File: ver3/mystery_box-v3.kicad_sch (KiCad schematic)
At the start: 3 parts, among them J1 Conn_01x02_Socket, Q1 IRLZ44N

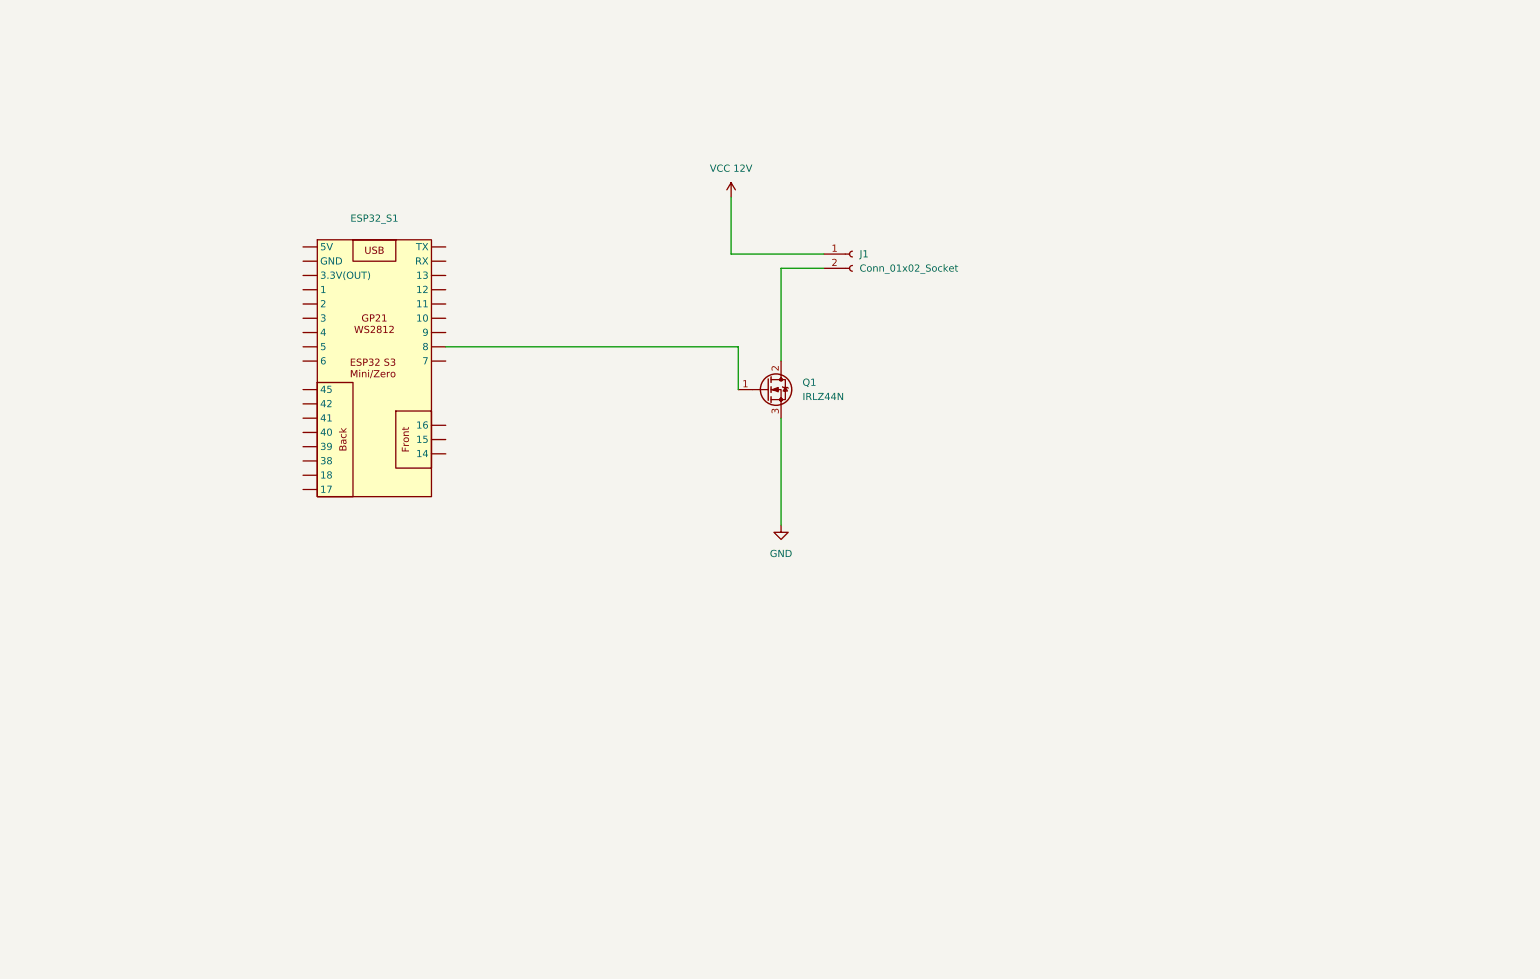
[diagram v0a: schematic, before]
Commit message: first draft v3
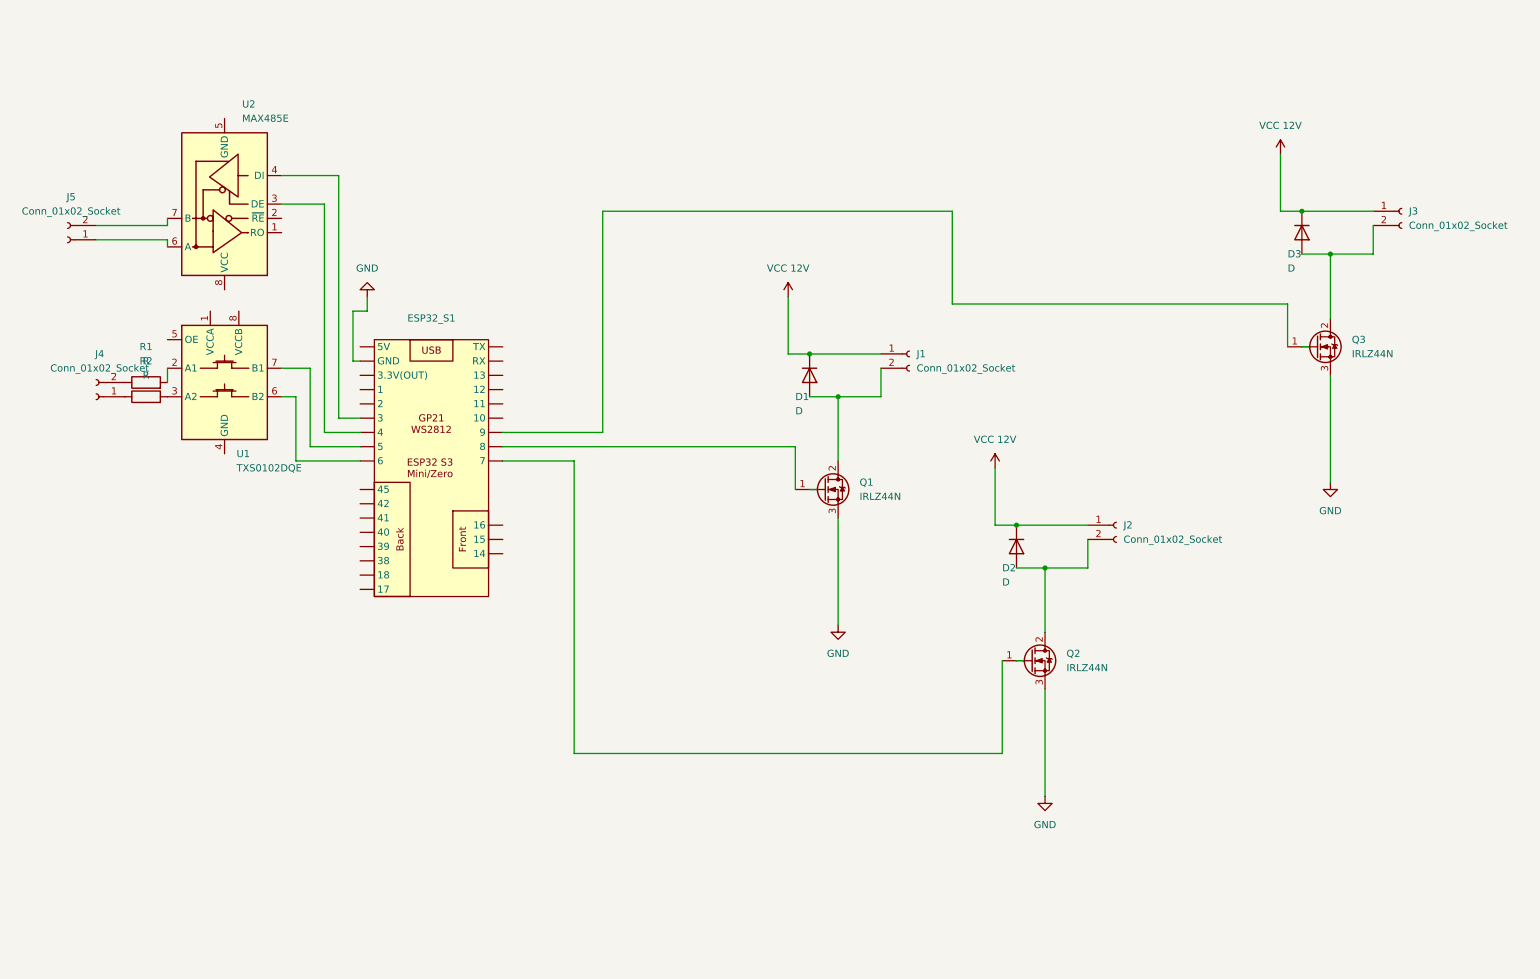
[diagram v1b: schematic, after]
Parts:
- added D1, D2, D3: D, symbol Device:D
- added J2, J3, J4, J5: Conn_01x02_Socket, symbol Connector:Conn_01x02_Socket
- added Q2, Q3: IRLZ44N, Package_TO_SOT_THT:TO-220-3_Vertical, symbol Transistor_FET:IRLZ44N
- added R1, R2: R, symbol Device:R
- added U1: TXS0102DQE, Package_SON:X2SON-8_1.4x1mm_P0.35mm, symbol Logic_LevelTranslator:TXS0102DQE
- added U2: MAX485E, Package_SO:SOIC-8_3.9x4.9mm_P1.27mm, symbol Interface_UART:MAX485E
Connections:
- net GND: now also ESP32_S1. (14), Q2.3 (S), Q3.3 (S)
- net VCC 12V: now also D1.1 (K), D2.1 (K), D3.1 (K), J2.1 (Pin_1), J3.1 (Pin_1)
- net at J1.2 (Pin_2), Q1.2 (D): now also D1.2 (A)
- new net: D3.2 (A), J3.2 (Pin_2), Q3.2 (D)
- new net: J4.1 (Pin_1), R2.1
- new net: R2.2, U1.3 (A2)
- new net: J4.2 (Pin_2), R1.1
- new net: R1.2, U1.2 (A1)
- new net: ESP32_S1. (14), Q2.1 (G)
- new net: ESP32_S1. (14), Q3.1 (G)
- new net: ESP32_S1. (14), U1.6 (B2)
- new net: ESP32_S1. (14), U1.7 (B1)
- new net: ESP32_S1. (14), U2.3 (DE)
- new net: ESP32_S1. (14), U2.4 (DI)
- new net: D2.2 (A), J2.2 (Pin_2), Q2.2 (D)
- new net: J5.1 (Pin_1), U2.6 (A)
- new net: J5.2 (Pin_2), U2.7 (B)
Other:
- moved on the sheet: ESP32_S1, J1, Q1

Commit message: update 2. meeting
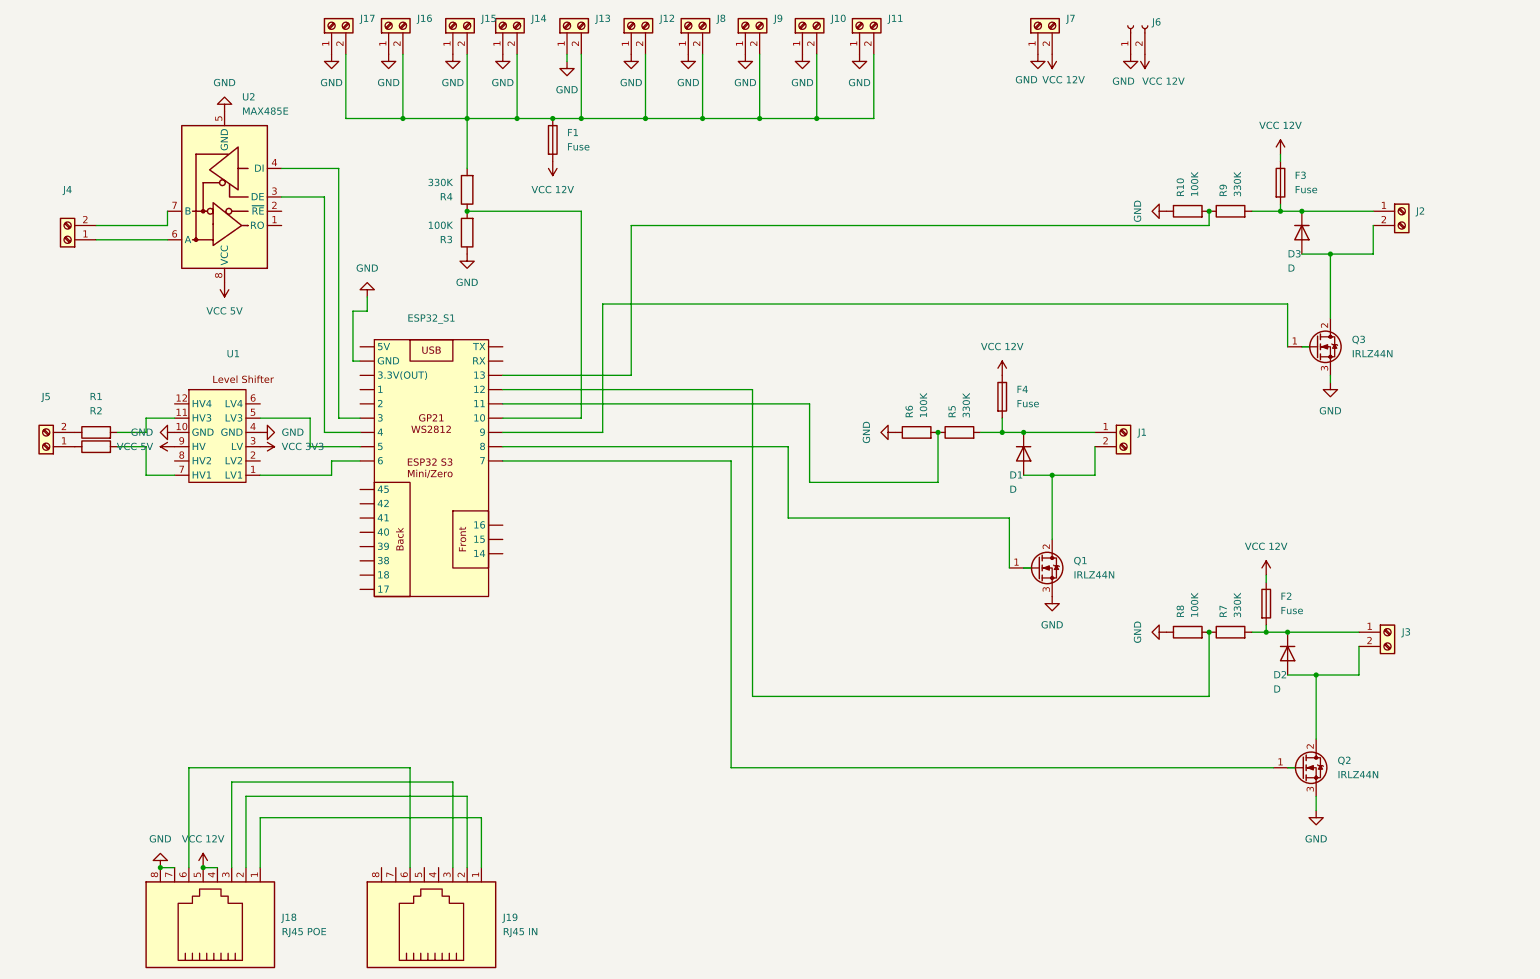
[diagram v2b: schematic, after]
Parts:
- removed J1, J2, J3, J4, J5: Conn_01x02_Socket, symbol Connector:Conn_01x02_Socket
- removed U1: TXS0102DQE, Package_SON:X2SON-8_1.4x1mm_P0.35mm, symbol Logic_LevelTranslator:TXS0102DQE
- added F1, F2, F3, F4: Fuse, symbol Device:Fuse
- added J1, J10, J11, J12, J13, J14, J15, J16, J17, J2, J3, J4, J5, J7, J8, J9: Screw_Terminal_01x02, symbol Connector:Screw_Terminal_01x02
- added J18: RJ45 POE, symbol Connector:RJ45
- added J19: RJ45 IN, symbol Connector:RJ45
- added J6: Conn_01x02_Socket, symbol Connector:Conn_01x02_Socket
- added R10, R3, R6, R8: 100K, symbol Device:R
- added R4, R5, R7, R9: 330K, symbol Device:R
- added U1: ~, eigene_footprints:level_shifter, symbol eigene:levelshifter_2channel
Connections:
- net GND: now also U2.5 (GND), J10.1 (Pin_1), J11.1 (Pin_1), J12.1 (Pin_1), J13.1 (Pin_1), J14.1 (Pin_1), J15.1 (Pin_1), J16.1 (Pin_1), J17.1 (Pin_1), J18.7, J18.8, J6.1 (Pin_1), J7.1 (Pin_1), J8.1 (Pin_1), J9.1 (Pin_1), R10.1, R3.1, R6.1, R8.1, U1.10 (GND), U1.4 (GND)
- net VCC 12V: now also F1.2, F2.1, F3.1, F4.1, J18.4, J18.5, J6.2 (Pin_2), J7.2 (Pin_2); no longer D1.1 (K), D2.1 (K), D3.1 (K)
- net at D3.2 (A), Q3.2 (D): now also J2.2 (Pin_2)
- net at R2.1: now also J5.1 (Pin_1)
- net at R2.2: now also U1.7 (HV1)
- net at R1.1: now also J5.2 (Pin_2)
- net at R1.2: now also U1.11 (HV3)
- net at D1.2 (A), Q1.2 (D): now also J1.2 (Pin_2)
- net at D2.2 (A), Q2.2 (D): now also J3.2 (Pin_2)
- net at U2.6 (A): now also J4.1 (Pin_1)
- net at U2.7 (B): now also J4.2 (Pin_2)
- net VCC 5V: now reaches U2.8 (VCC)
- net VCC 5V: now also U1.9 (HV)
- new net: ESP32_S1. (14), R7.1, R8.2
- new net: D2.1 (K), F2.2, J3.1 (Pin_1), R7.2
- new net: ESP32_S1. (14), R10.2, R9.1
- new net: F1.1, J10.2 (Pin_2), J11.2 (Pin_2), J12.2 (Pin_2), J13.2 (Pin_2), J14.2 (Pin_2), J15.2 (Pin_2), J16.2 (Pin_2), J17.2 (Pin_2), J8.2 (Pin_2), J9.2 (Pin_2), R4.2
- new net: J18.1, J19.1
- new net: J18.2, J19.2
- new net: J18.3, J19.3
- new net: J18.6, J19.6
- new net: D1.1 (K), F4.2, J1.1 (Pin_1), R5.2
- new net: D3.1 (K), F3.2, J2.1 (Pin_1), R9.2
- new net: ESP32_S1. (14), R5.1, R6.2
- new net: ESP32_S1. (14), U1.1 (LV1)
- new net: ESP32_S1. (14), U1.5 (LV3)
- new net: ESP32_S1. (14), R3.2, R4.1
- new net VCC 3V3: U1.3 (LV)
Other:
- moved on the sheet: D1, D2, Q1, Q2, R1, R2, U2
